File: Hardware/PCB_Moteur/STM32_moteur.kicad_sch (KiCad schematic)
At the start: 66 parts, among them J2 Conn_01x06_Pin, U2 STM32F103CBT6

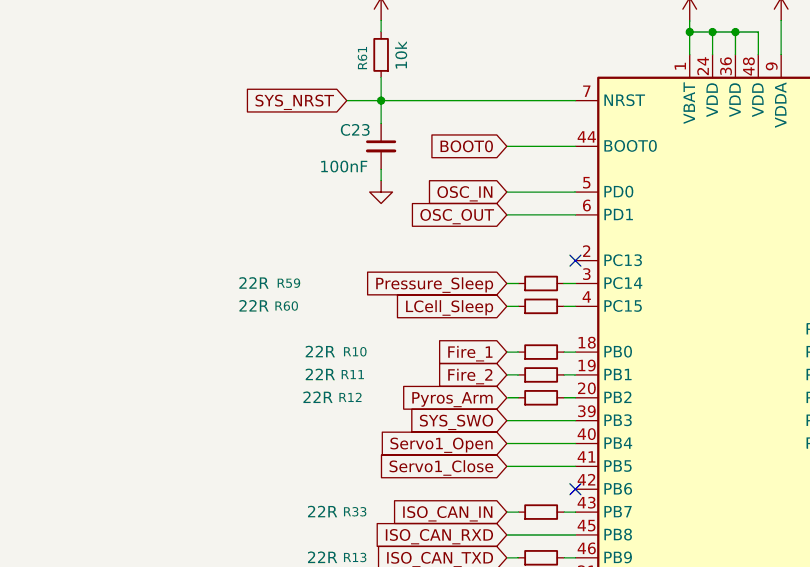
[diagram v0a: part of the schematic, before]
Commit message: wip: new pressure et fix alim
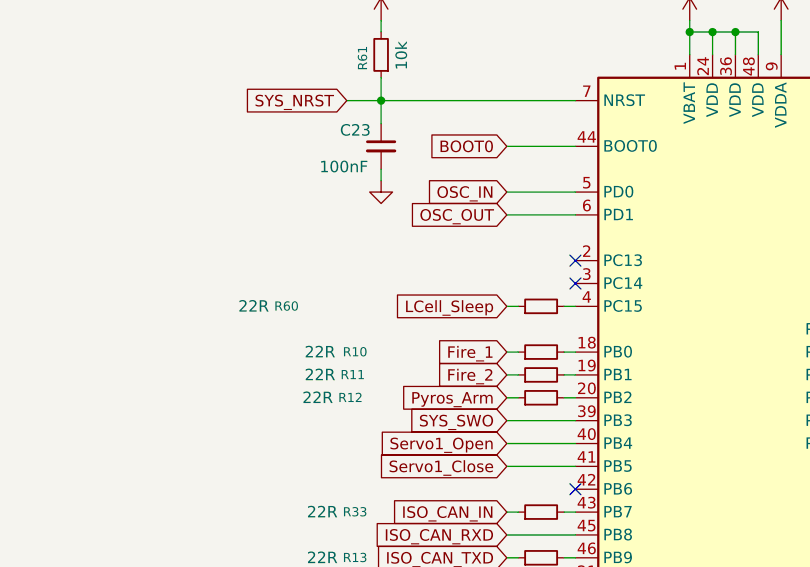
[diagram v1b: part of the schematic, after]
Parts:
- removed R59: 22R, Resistor_SMD:R_0603_1608Metric, symbol Device:R_Small
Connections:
- no-connect marks 2 -> 3
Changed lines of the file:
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@@
 	)
 	(no_connect
+		(at 133.35 72.39)
+	)
+	(no_connect
 		(at 133.35 95.25)
 	)
@@
 	(wire
 		(pts
-			(xy 125.73 72.39) (xy 127 72.39)
-		)
-		(stroke
-			(width 0)
-			(type default)
-		)
-	)
-	(wire
-		(pts
 			(xy 243.84 35.56) (xy 251.46 35.56)
 		)
@@
 	(wire
 		(pts
-			(xy 132.08 72.39) (xy 133.35 72.39)
-		)
-		(stroke
-			(width 0)
-			(type default)
-		)
-	)
-	(wire
-		(pts
 			(xy 148.59 127) (xy 151.13 127)
 		)
@@
 		)
 	)
-	(global_label "Pressure_Sleep"
-		(shape input)
-		(at 125.73 72.39 180)
-		(fields_autoplaced yes)
-		(effects
-			(font
-				(size 1.27 1.27)
-			)
-			(justify right)
-		)
-		(property "Intersheetrefs" "${INTERSHEET_REFS}"
-			(at 108.3515 72.39 0)
-			(effects
-				(font
-					(size 1.27 1.27)
-				)
-				(justify right)
-				(hide yes)
-			)
-		)
-	)
 	(global_label "Servo3_Close"
 		(shape input)
@@
 					(unit 1)
 				)
-			)
-		)
-	)
-	(symbol
-		(lib_id "Device:R_Small")
-		(at 129.54 72.39 90)
-		(unit 1)
-		(exclude_from_sim no)
-		(in_bom yes)
-		(on_board yes)
-		(dnp no)
-		(property "Reference" "R59"
-			(at 102.87 72.39 90)
-			(effects
-				(font
-					(size 1.016 1.016)
-				)
-				(justify left)
-			)
-		)
-		(property "Value" "22R"
-			(at 99.314 72.39 90)
-			(effects
-				(font
-					(size 1.27 1.27)
-				)
-				(justify left)
-			)
-		)
-		(property "Footprint" "Resistor_SMD:R_0603_1608Metric"
-			(at 129.54 72.39 0)
-			(effects
-				(font
-					(size 1.27 1.27)
-				)
-				(hide yes)
-			)
-		)
-		(property "Datasheet" "~"
-			(at 129.54 72.39 0)
-			(effects
-				(font
-					(size 1.27 1.27)
-				)
-				(hide yes)
-			)
-		)
-		(property "Description" "Resistor, small symbol"
-			(at 129.54 72.39 0)
-			(effects
-				(font
-					(size 1.27 1.27)
-				)
-				(hide yes)
-			)
-		)
-		(pin "1"
-		)
-		(pin "2"
-		)
-		(instances
-			(project "PCB_moteur"
-				(path "/b0d87684-7b1c-41d8-8358-755aa327573e/753d1783-c2f5-4012-bbb8-3f4eadf066f6"
-					(reference "R59")
-					(unit 1)
-				)
-			)
-			(project "STM32_moteur"
-				(path "/da6e3e70-7434-4a0f-acc5-62316b7258e2"
-					(reference "R?")
-					(unit 1)
-				)
